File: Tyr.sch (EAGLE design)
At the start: 206 parts, among them J1 TYR_TYR_DISPLAY, Q1 DTC123J, SW1 BUTTON, U1 MCP1700T, U2 CONTROLLER_PRTR5V0U2X, U3 STM32F303CC, U4 MB85RC256V, U6 TYR_TPS2552, X1 CONTROLLER_USB-C-12PUSB-C-12P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, Y1 8Mhz

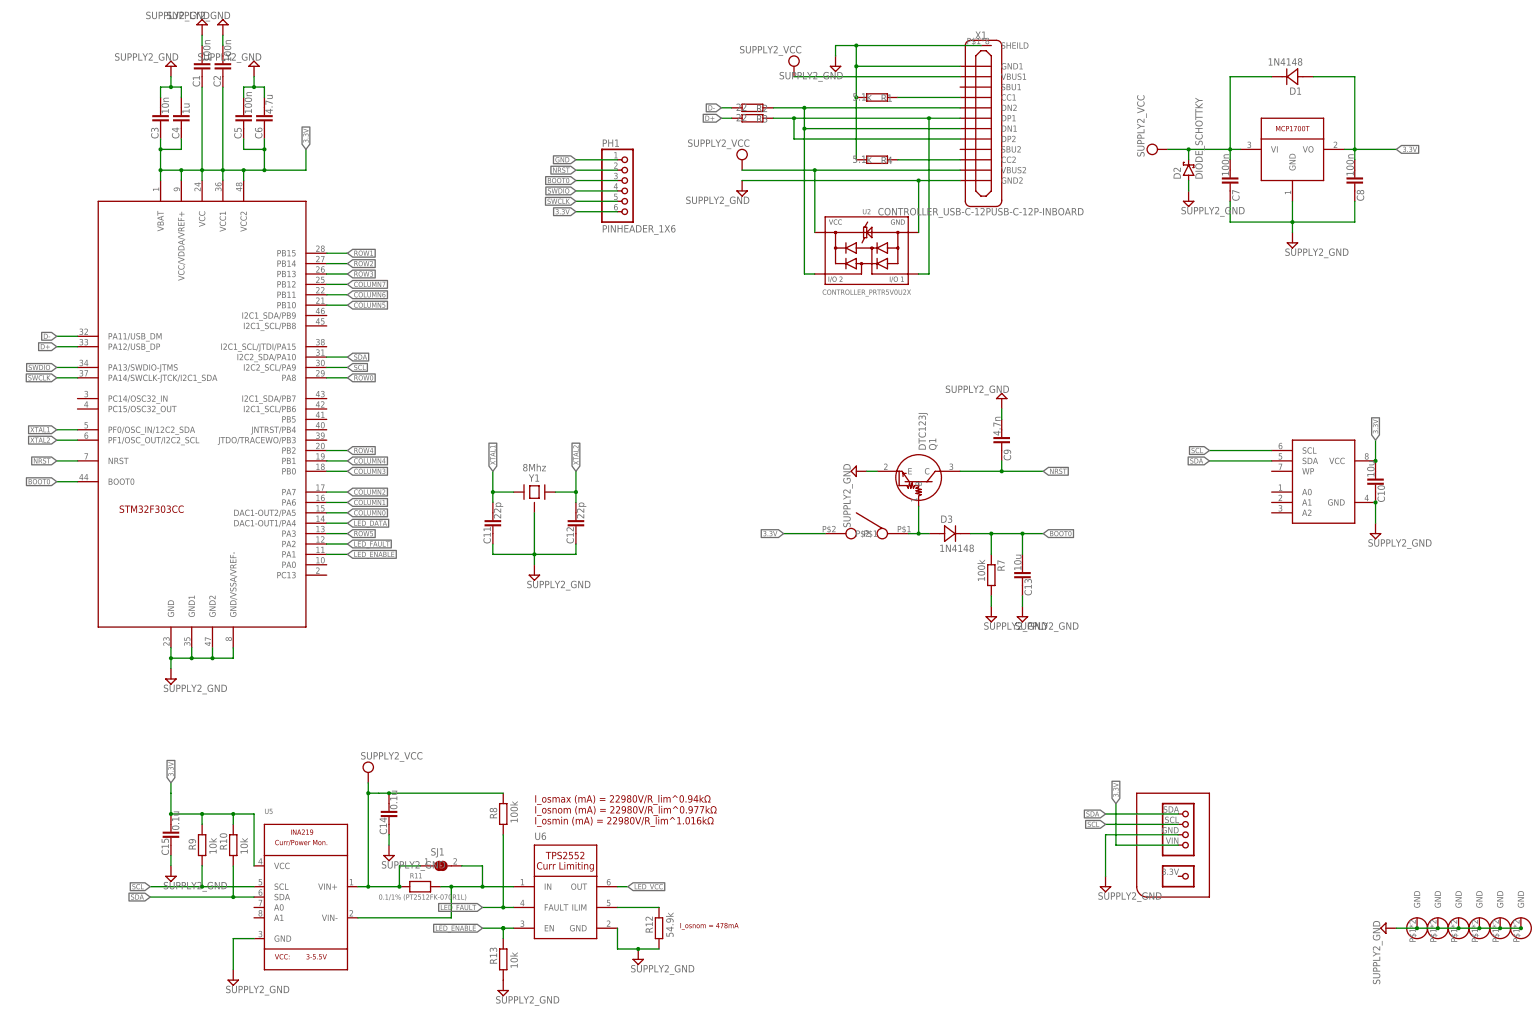
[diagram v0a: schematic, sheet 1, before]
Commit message: Update logo
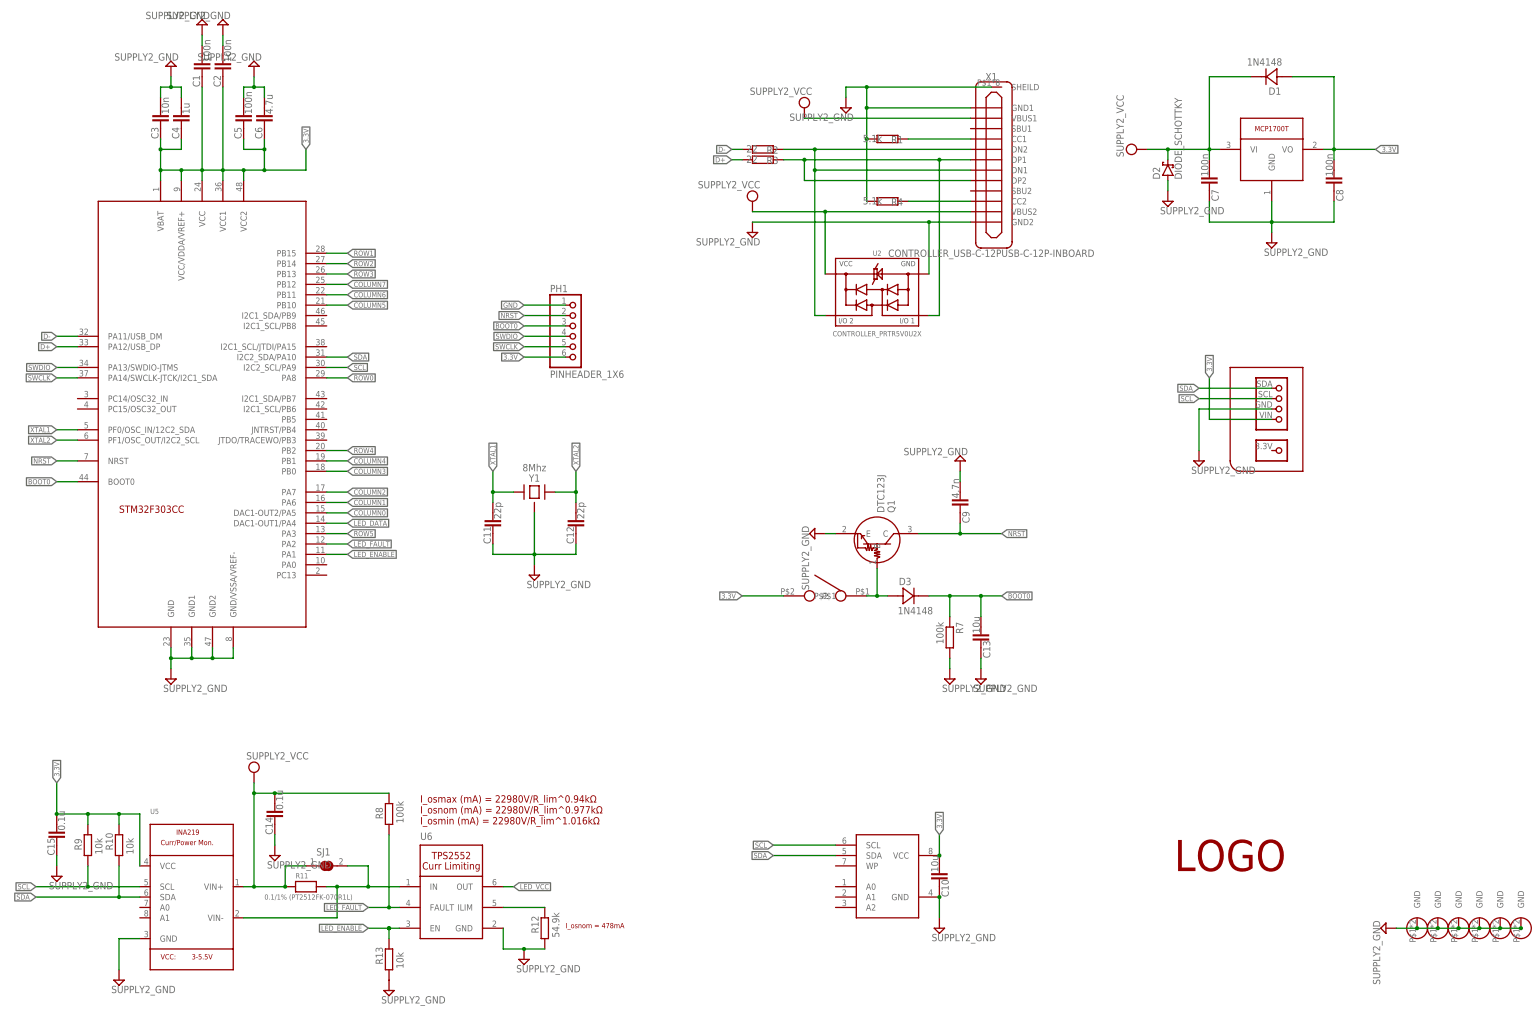
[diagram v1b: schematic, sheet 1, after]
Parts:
- added U$1: LOGO_TYR, Tyr:LOGO_TYR
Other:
- note added: "5V to 3.3V Regulator"
- note added: "DFU Hard Reset Circuit"
- note added: "I2C FRAM Module"
- note added: "MCU & Crystal"
- note added: "RGB Current Monitoring & Limiting"
- note added: "Type-C & ESD Protection"
- moved on the sheet: C10, C13, C14, C15, C7, C8, C9, D1, D2, D3, PH1, Q1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
